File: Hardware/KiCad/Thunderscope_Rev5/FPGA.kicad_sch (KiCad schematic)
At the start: 40 parts, among them J5 2.54mm 6 Pin TH

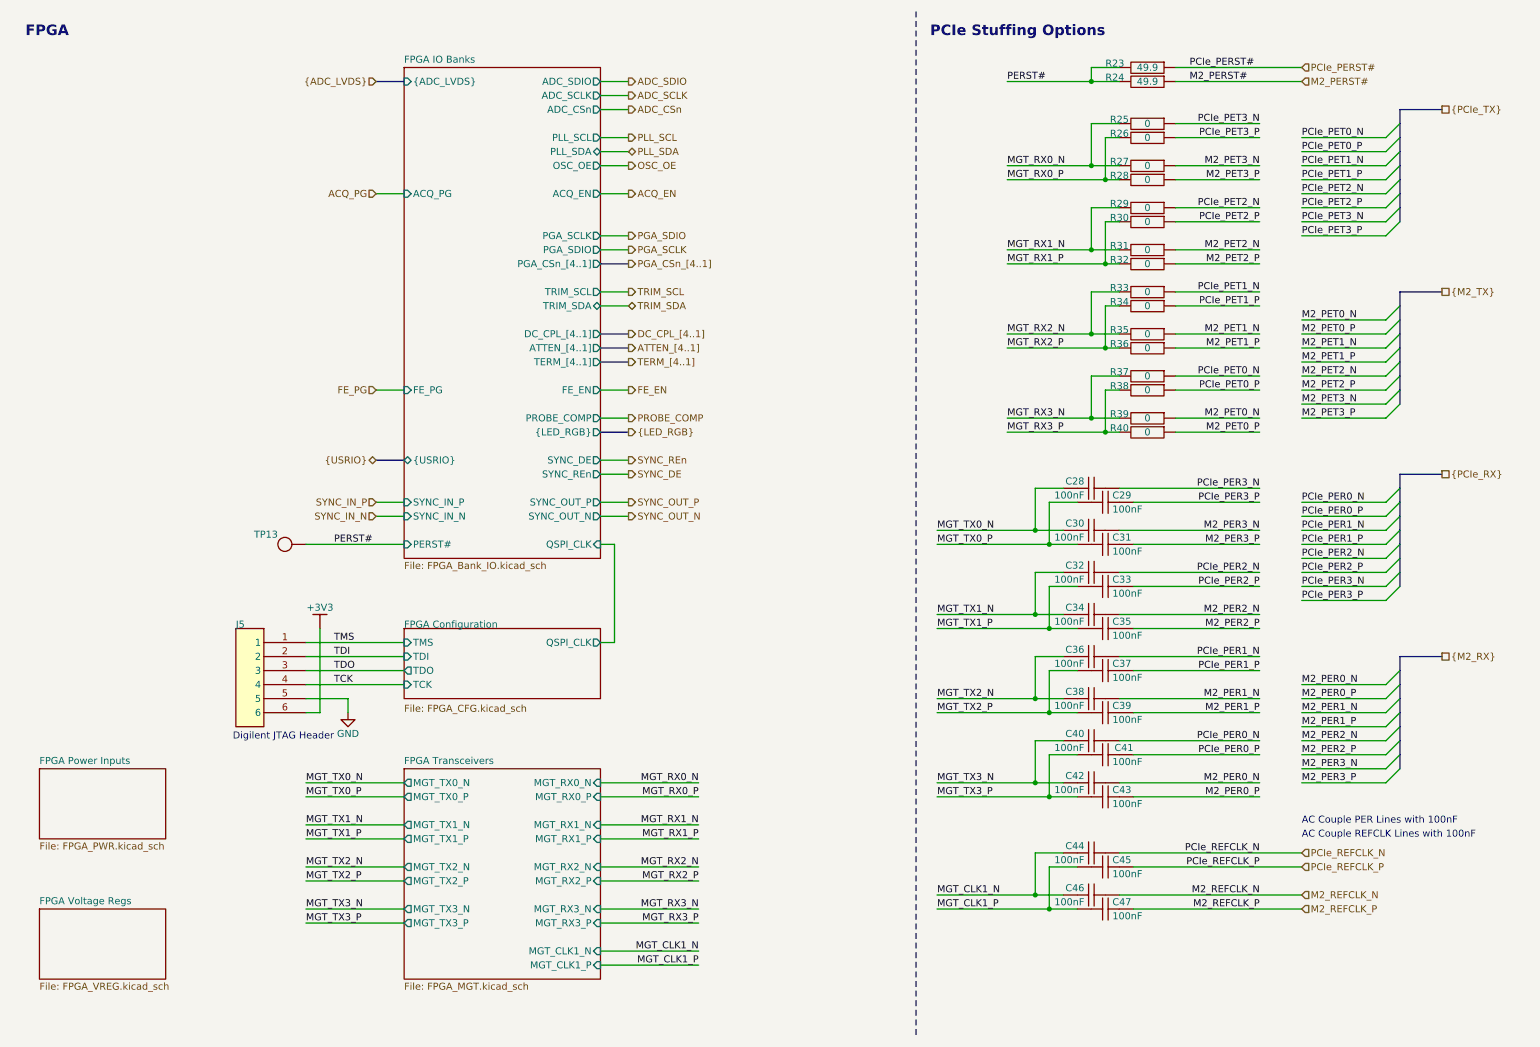
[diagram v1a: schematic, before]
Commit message: Refactored Schematic
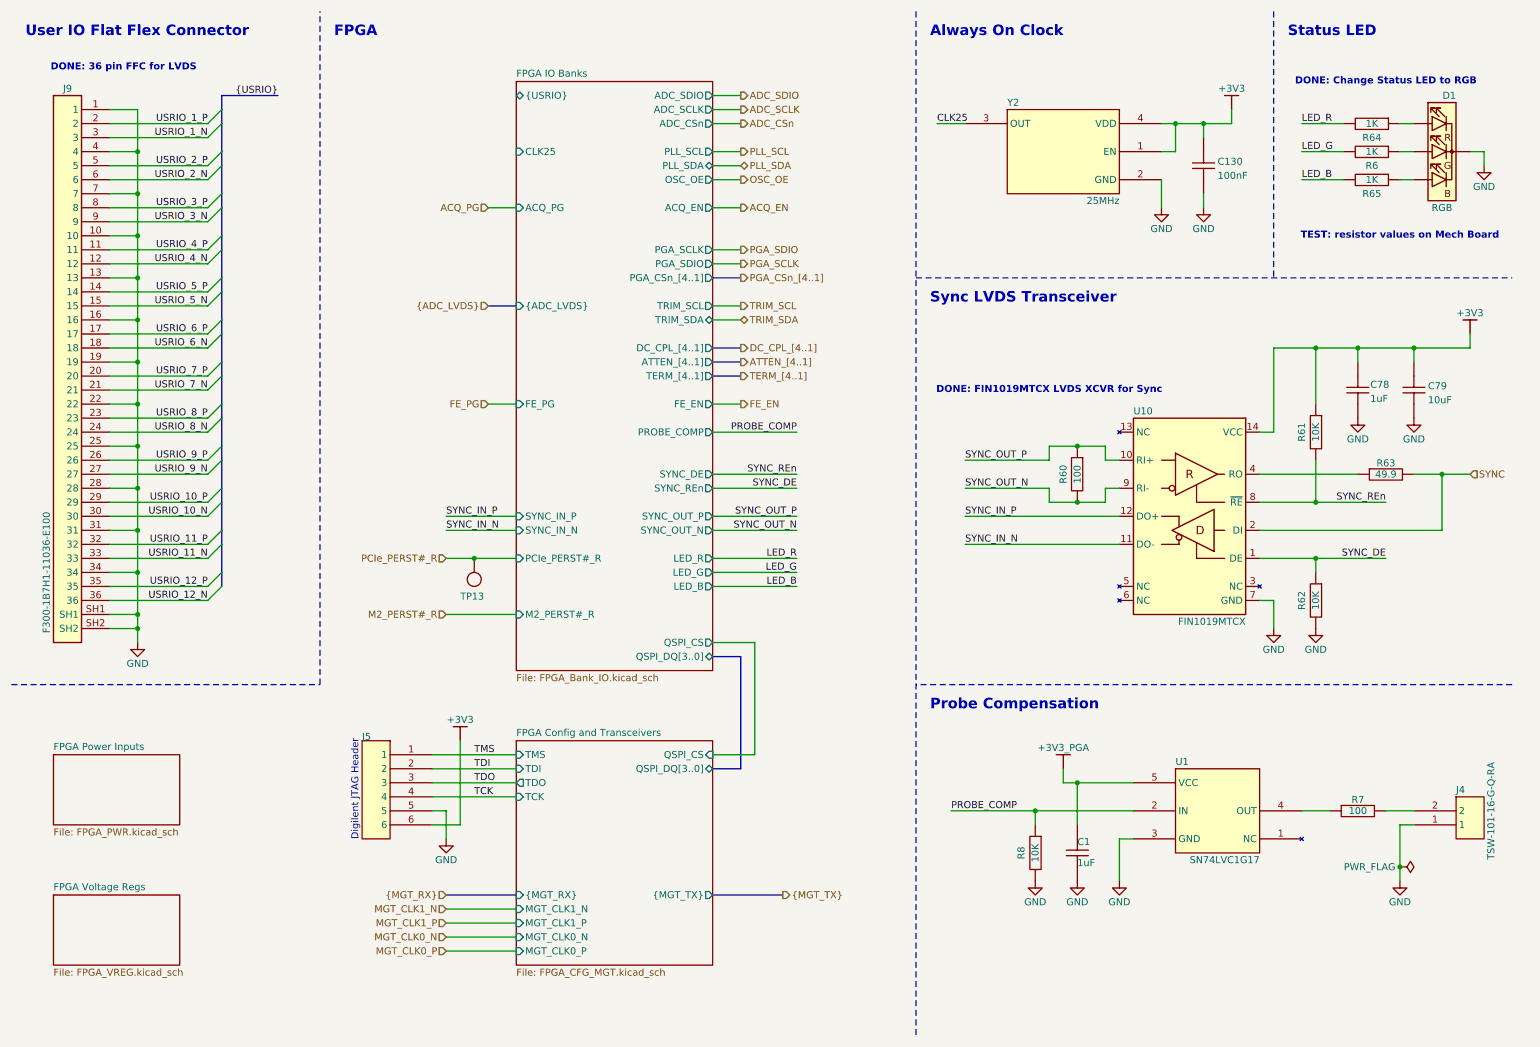
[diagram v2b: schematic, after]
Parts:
- removed C28, C29, C30, C31, C32, C33, C34, C35, C36, C37, C38, C39, C40, C41, C42, C43, C44, C45, C46, C47: 100nF, Thunderscope_Rev5:GEN_C_0201, symbol Thunderscope_Rev5:CAP 100nF 6.3V X5R 0201
- removed R23, R24: 49.9, Thunderscope_Rev5:GEN_R_0402, symbol Thunderscope_Rev5:RES 49.9 OHM 1% 1/10W 0402
- removed R25, R26, R27, R28, R29, R30, R31, R32, R33, R34, R35, R36, R37, R38, R39, R40: 0, Thunderscope_Rev5:GEN_R_0201, symbol Thunderscope_Rev5:RES 0 OHM 1% 1/20W 0201
- added C1, C78: 1uF, Thunderscope_Rev5:GEN_C_0402, symbol Thunderscope_Rev5:CAP 1uF 25V X5R 0402
- added C130: 100nF, Thunderscope_Rev5:GEN_C_0402, symbol Thunderscope_Rev5:CAP 100nF 16V X7R 0402
- added C79: 10uF, Thunderscope_Rev5:GEN_C_0603, symbol Thunderscope_Rev5:CAP 10uF 10V X5R 0603
- added D1: RGB, Thunderscope_Rev5:LED_Kingbright_APFA3010_3x1.5mm_Horizontal, symbol Thunderscope_Rev5:LED RGB 1204 APFA3010LSEKJ3ZGKQBC
- added J4: TSW-101-16-G-Q-RA, Thunderscope_Rev5:GEN_5.08mm_1x2_Pin_TH_RA, symbol Thunderscope_Rev5:CONN 5.08mm 2 Pin TH RA
- added J9: F300-1B7H1-11036-E100, Thunderscope_Rev5:AMPHENOL_F300-1B7H1-11036-E100, symbol Thunderscope_Rev5:CONN FFC BOTTOM 36POS 0.5MM RA
- added R6, R64, R65: 1K, Thunderscope_Rev5:GEN_R_0402, symbol Thunderscope_Rev5:RES 1K OHM 1% 1/10W 0402
- added R60, R7: 100, Thunderscope_Rev5:GEN_R_0402, symbol Thunderscope_Rev5:RES 100 OHM 1% 1/10W 0402
- added R61, R62, R8: 10K, Thunderscope_Rev5:GEN_R_0402, symbol Thunderscope_Rev5:RES 10K OHM 1% 1/10W 0402
- added R63: 49.9, Thunderscope_Rev5:GEN_R_0402, symbol Thunderscope_Rev5:RES 49.9 OHM 1% 1/10W 0402
- added U1: SN74LVC1G17, Thunderscope_Rev5:GEN_SC-70-5, symbol Thunderscope_Rev5:IC BUFFER SN74LVC1G17
- added U10: FIN1019MTCX, Thunderscope_Rev5:GEN_TSSOP-14_4.4x5mm_P0.65mm, symbol Thunderscope_Rev5:IC LVDS XCVR FIN1019MTCX
- added Y2: 25MHz, Thunderscope_Rev5:ECS_TXO-2016, symbol Thunderscope_Rev5:OSC 25MHz ECS-TXO-2016
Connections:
- net +3V3: now also C130.2, C78.1, C79.2, R61.1, U10.14 (VCC), Y2.1 (EN), Y2.4 (VDD)
- net GND: now also C1.2, C130.1, C78.2, C79.1, D1.2 (A), J4.1, J9.1, J9.10, J9.13, J9.16, J9.19, J9.22, J9.25, J9.28, J9.31, J9.34, J9.4, J9.7, J9.SH1, J9.SH2, R62.2, R8.2, U1.3 (GND), U10.7 (GND), Y2.2 (GND)
- net PROBE_COMP: now also R8.1, U1.2 (IN)
- net SYNC_DE: now also R62.1, U10.1 (DE)
- net SYNC_IN_N: now also U10.11 (DO-)
- net SYNC_IN_P: now also U10.12 (DO+)
- net SYNC_OUT_N: now also R60.1, U10.9 (RI-)
- net SYNC_OUT_P: now also R60.2, U10.10 (RI+)
- net SYNC_REn: now also R61.2, U10.8 (~{RE})
- net PERST# renamed PCIe_PERST#_R
- new net: D1.1 (R), R64.1
- new net: D1.3 (G), R6.1
- new net: D1.4 (B), R65.1
- new net: R63.2, U10.4 (RO)
- new net: R7.2, U1.4 (OUT)
- new net: J4.2, R7.1
- new net +3V3_PGA: C1.1, U1.5 (VCC)
- new net CLK25: Y2.3 (OUT)
- new net LED_B: R65.2
- new net LED_G: R6.2
- new net LED_R: R64.2
- new net SYNC: R63.1, U10.2 (DI)
- new net USRIO_10_N: J9.30
- new net USRIO_10_P: J9.29
- new net USRIO_11_N: J9.33
- new net USRIO_11_P: J9.32
- new net USRIO_12_N: J9.36
- new net USRIO_12_P: J9.35
- new net USRIO_1_N: J9.3
- new net USRIO_1_P: J9.2
- new net USRIO_2_N: J9.6
- new net USRIO_2_P: J9.5
- new net USRIO_3_N: J9.9
- new net USRIO_3_P: J9.8
- new net USRIO_4_N: J9.12
- new net USRIO_4_P: J9.11
- new net USRIO_5_N: J9.15
- new net USRIO_5_P: J9.14
- new net USRIO_6_N: J9.18
- new net USRIO_6_P: J9.17
- new net USRIO_7_N: J9.21
- new net USRIO_7_P: J9.20
- new net USRIO_8_N: J9.24
- new net USRIO_8_P: J9.23
- new net USRIO_9_N: J9.27
- new net USRIO_9_P: J9.26
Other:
- sheet FPGA Configuration renamed FPGA Config and Transceivers
- removed sheet FPGA Transceivers
- sheet FPGA Config and Transceivers: file FPGA_CFG.kicad_sch -> FPGA_CFG_MGT.kicad_sch
- sheet FPGA Config and Transceivers ports: added MGT_CLK0_N, MGT_CLK0_P, MGT_CLK1_N, MGT_CLK1_P, QSPI_CS, QSPI_DQ[3..0], {MGT_RX}, {MGT_TX}; removed QSPI_CLK
- sheet FPGA IO Banks ports: added CLK25, LED_B, LED_G, LED_R, M2_PERST#_R, PCIe_PERST#_R, QSPI_CS, QSPI_DQ[3..0]; removed PERST#, QSPI_CLK, {LED_RGB}
- note added: "Always On Clock"
- note added: "DONE: 36 pin FFC for LVDS"
- note added: "DONE: Change Status LED to RGB"
- note added: "DONE: FIN1019MTCX LVDS XCVR for Sync"
- note added: "Probe Compensation"
- note added: "Status LED"
- note added: "Sync LVDS Transceiver"
- note added: "TEST: resistor values on Mech Board"
- note added: "User IO Flat Flex Connector"
- note removed: "AC Couple PER Lines with 100nF"
- note removed: "AC Couple REFCLK Lines with 100nF"
- note removed: "PCIe Stuffing Options"
- moved on the sheet: J5, TP13
